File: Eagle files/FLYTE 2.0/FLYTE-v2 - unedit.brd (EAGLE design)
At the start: 116 x 55 mm, 58 parts, among them U2 XBP9B-XCST-021, U3 ADS1115IDGSR, U4 H3LIS200DLTR, U5 BS170F, U6 W25Q32JVSSIQ, U7 BS170F

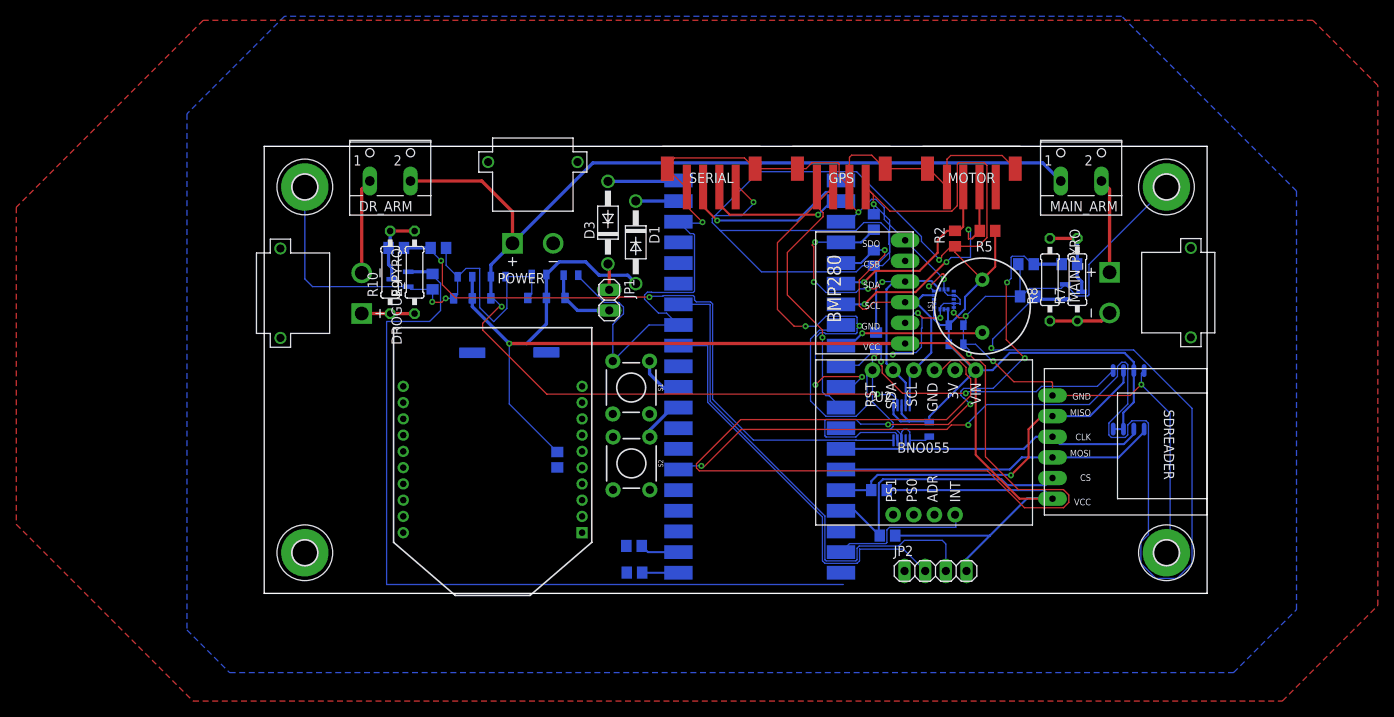
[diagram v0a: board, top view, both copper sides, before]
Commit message: routing done
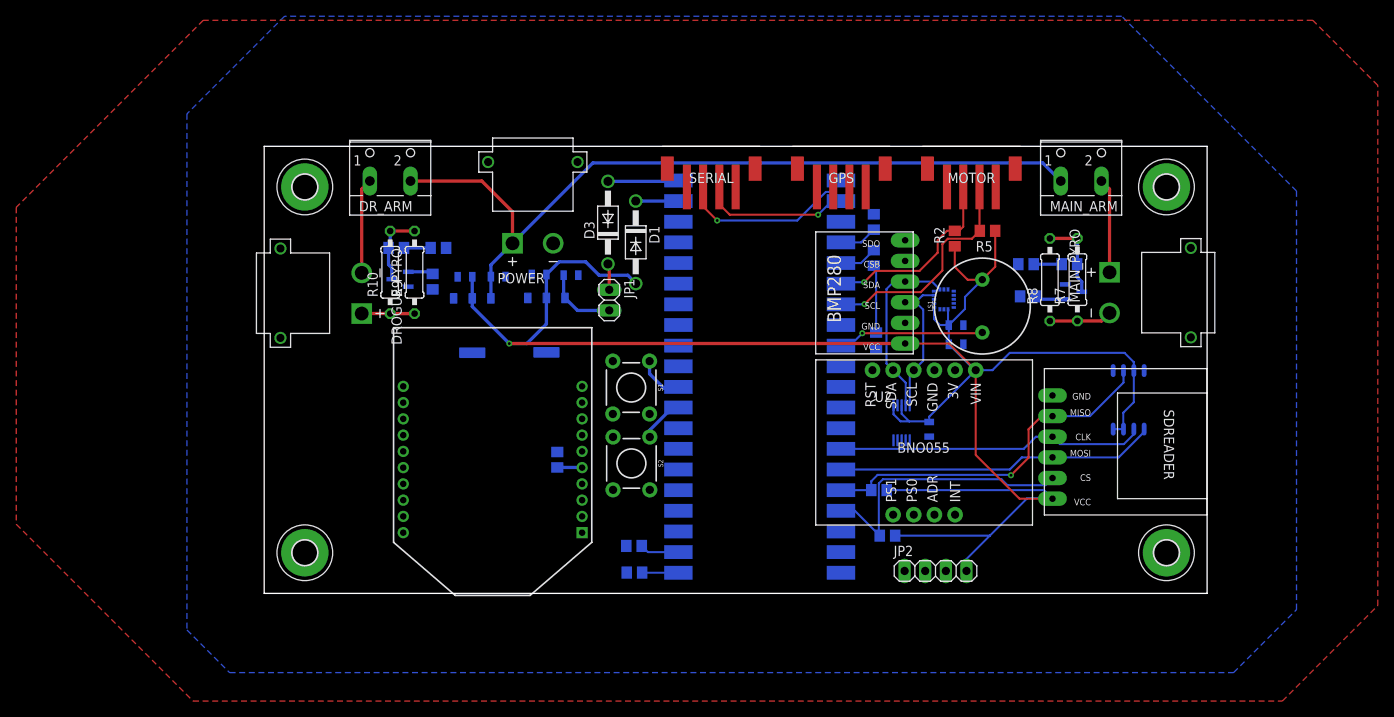
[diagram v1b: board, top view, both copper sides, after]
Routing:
- net GND: track 497.4 -> 0.00 mm, vias 15 -> 0
- net 3V3: track 415.3 -> 252.7 mm, vias 4 -> 1
- net MAIN: track 163.7 -> 4.40 mm, vias 3 -> 0
- net DROGUE: track 103.7 -> 3.10 mm
- net SENSE_DROG: track 79.3 -> 3.28 mm, vias 2 -> 0
- net AIR_DATA: track 61.5 -> 0.00 mm
- net VCC: track 159.6 -> 98.3 mm, vias 2 -> 0
- net SENSE_MAIN: track 63.2 -> 3.44 mm, vias 4 -> 0
- net TX: track 52.0 -> 0.00 mm, vias 4 -> 0
- net AIR_SCK: track 51.3 -> 0.00 mm
- net CS_FLASH: track 39.3 -> 0.00 mm, vias 2 -> 0
- net RX: track 32.2 -> 0.00 mm, vias 1 -> 0
- net SDA1: track 48.1 -> 27.3 mm, vias 4 -> 0
- net BNO_INT: track 17.9 -> 0.00 mm
- net SCL1: track 38.8 -> 22.4 mm, vias 1 -> 0
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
